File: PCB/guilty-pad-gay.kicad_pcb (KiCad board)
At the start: 2 copper layers, 6 parts

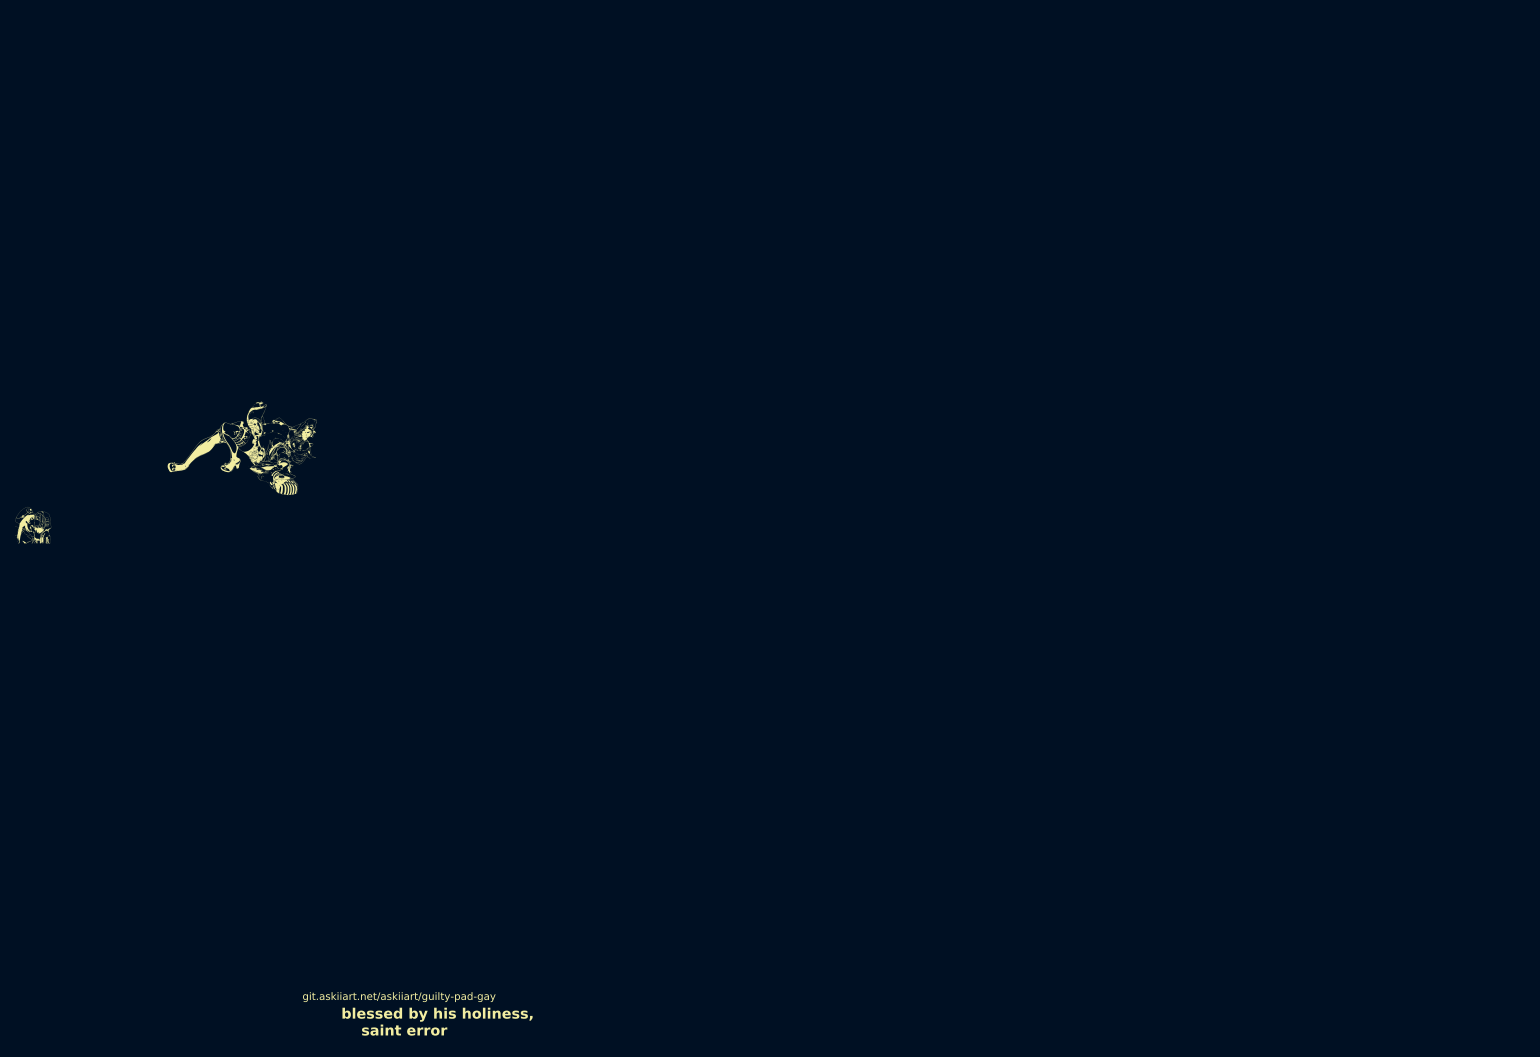
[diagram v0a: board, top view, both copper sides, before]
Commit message: update with routed and parts and stuffs
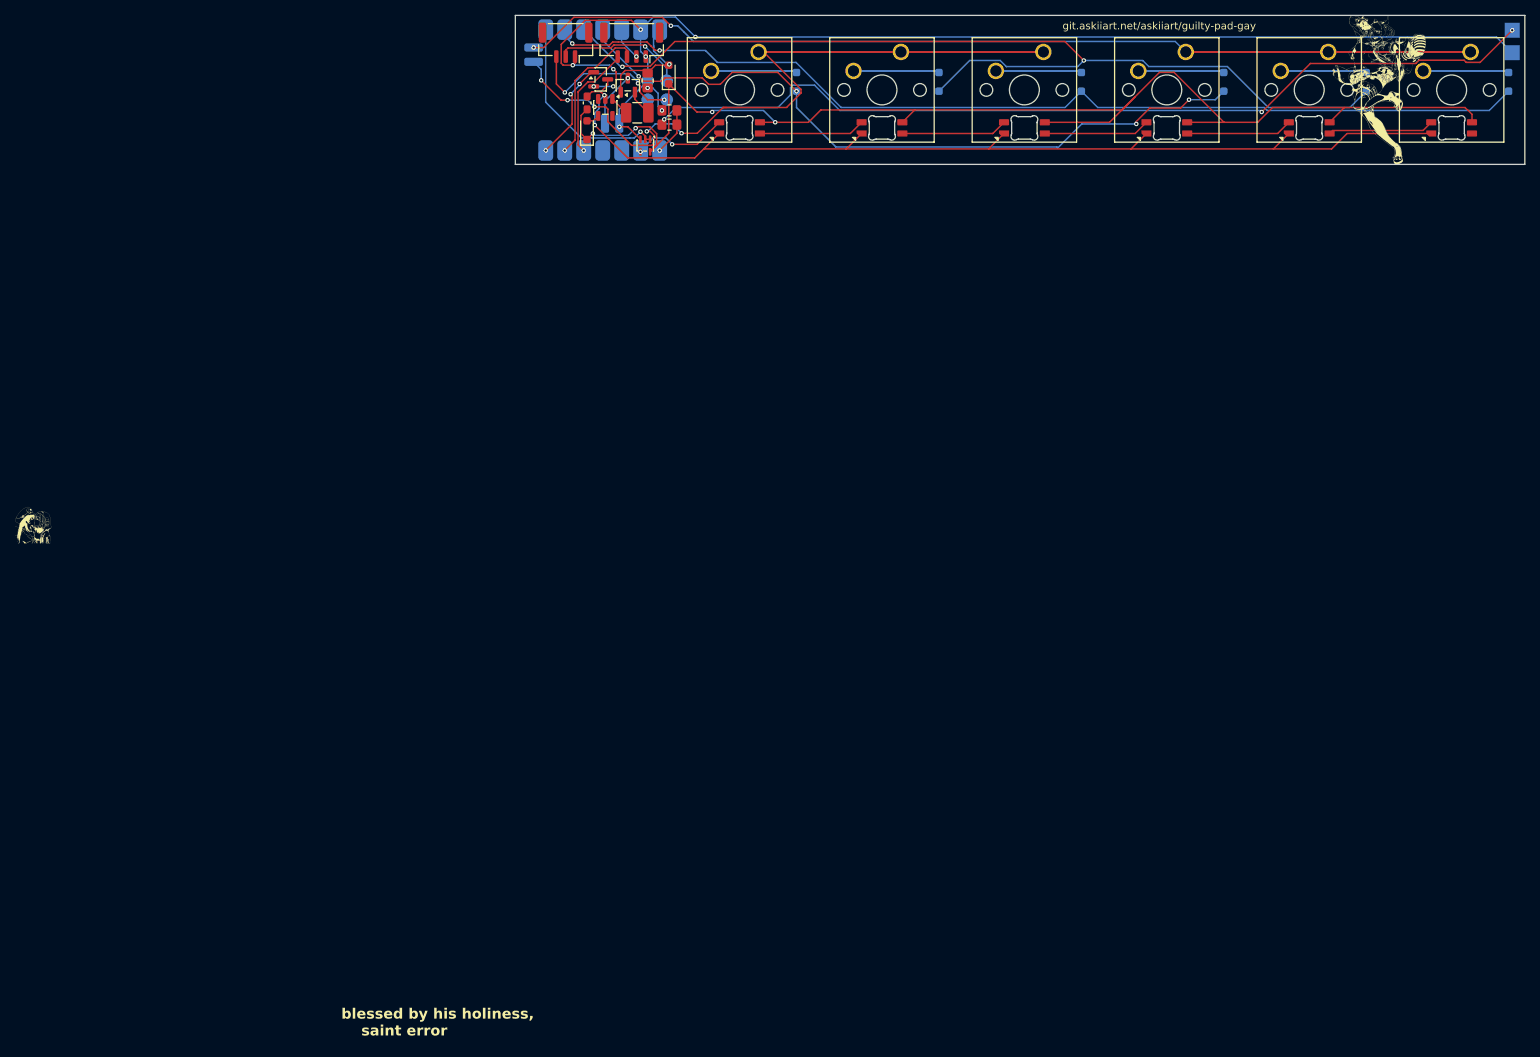
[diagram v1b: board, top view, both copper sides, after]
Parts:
- added C2: 22uF, Capacitor_SMD:C_0603_1608Metric_Pad1.08x0.95mm_HandSolder, F.Cu at (116.0, 70.8)
- added D1: D, Diode_SMD:D_SOD-323_HandSoldering, F.Cu at (116.0, 74.4)
- added D2: D, Diode_SMD:D_SOD-323_HandSoldering, F.Cu at (126.9, 67.0)
- added D3: D_Small, Diode_SMD:D_SOD-323_HandSoldering, B.Cu at (144.0, 68.0)
- added D4: D_Small, Diode_SMD:D_SOD-323_HandSoldering, B.Cu at (201.2, 68.0)
- added D5: D_Small, Diode_SMD:D_SOD-323_HandSoldering, B.Cu at (163.1, 68.0)
- added D6: D_Small, Diode_SMD:D_SOD-323_HandSoldering, B.Cu at (220.2, 68.0)
- added D7: D_Small, Diode_SMD:D_SOD-323_HandSoldering, B.Cu at (182.1, 68.0)
- added D8: D_Small, Diode_SMD:D_SOD-323_HandSoldering, B.Cu at (239.3, 68.0)
- added J1: Conn_01x03, Connector_JST:JST_GH_SM03B-GHS-TB_1x03-1MP_P1.25mm_Horizontal, F.Cu at (113.2, 62.7)
- added J2: Conn_01x04, Connector_JST:JST_GH_SM04B-GHS-TB_1x04-1MP_P1.25mm_Horizontal, F.Cu at (122.0, 62.7)
- added L1: 4.7uH, Inductor_SMD:L_1210_3225Metric_Pad1.42x2.65mm_HandSolder, F.Cu at (122.7, 72.1)
- added LED1: SK6812MINI-E, marbastlib-various:LED_6028R, F.Cu at (136.4, 74.1)
- added LED2: SK6812MINI-E, marbastlib-various:LED_6028R, F.Cu at (155.5, 74.1)
- added LED3: SK6812MINI-E, marbastlib-various:LED_6028R, F.Cu at (174.5, 74.1)
- added LED4: SK6812MINI-E, marbastlib-various:LED_6028R, F.Cu at (193.6, 74.1)
- added LED5: SK6812MINI-E, marbastlib-various:LED_6028R, F.Cu at (212.6, 74.1)
- added LED6: SK6812MINI-E, marbastlib-various:LED_6028R, F.Cu at (231.7, 74.1)
- added Q1: AO3400A, Package_TO_SOT_SMD:SOT-23, F.Cu at (117.8, 67.6)
- added Q2: AO3401A, Package_TO_SOT_SMD:SOT-23, F.Cu at (121.5, 68.4)
- added R1: 806k, Resistor_SMD:R_0805_2012Metric_Pad1.20x1.40mm_HandSolder, F.Cu at (127.0, 73.7)
- added R2: 2M, Resistor_SMD:R_0805_2012Metric_Pad1.20x1.40mm_HandSolder, F.Cu at (127.0, 71.8)
- added R3: 806k, Resistor_SMD:R_0805_2012Metric_Pad1.20x1.40mm_HandSolder, F.Cu at (124.1, 67.8)
- added SW1: SW_Push, Button_Switch_Keyboard:SW_Cherry_MX_1.00u_PCB, F.Cu at (138.9, 64.0)
- added SW2: SW_Push, Button_Switch_Keyboard:SW_Cherry_MX_1.00u_PCB, F.Cu at (158.0, 64.0)
- added SW3: SW_Push, Button_Switch_Keyboard:SW_Cherry_MX_1.00u_PCB, F.Cu at (177.0, 64.0)
- added SW4: SW_Push, Button_Switch_Keyboard:SW_Cherry_MX_1.00u_PCB, F.Cu at (196.1, 64.0)
- added SW5: SW_Push, Button_Switch_Keyboard:SW_Cherry_MX_1.00u_PCB, F.Cu at (215.1, 64.0)
- added SW6: SW_Push, Button_Switch_Keyboard:SW_Cherry_MX_1.00u_PCB, F.Cu at (234.2, 64.0)
- added TP1: TestPoint, TestPoint:TestPoint_Pad_2.0x2.0mm, B.Cu at (239.8, 61.1)
- added TP2: TestPoint, TestPoint:TestPoint_Pad_2.0x2.0mm, B.Cu at (239.8, 64.1)
- added U1: XIAO-nRF52840-SMD, OPL:XIAO-nRF52840-SMD, B.Cu at (118.1, 69.0)
- added U2: TPS613222ADBV, Package_TO_SOT_SMD:SOT-23-5, F.Cu at (118.4, 71.4)
- added U3: 74LV1T08GW, Package_TO_SOT_SMD:SOT-353_SC-70-5, F.Cu at (123.8, 76.5)
- moved G*** 159.8 mm to (222.2, 69.0), turned to 0 degrees
- moved G*** 120.2 mm to (187.7, 72.7)
- moved G*** 53.4 mm to (149.1, 73.7)
- moved G*** 44.7 mm to (165.4, 69.9), turned to 0 degrees
- moved G*** 37.4 mm to (113.2, 68.6), turned to 90 degrees
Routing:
- net /COL1: track 0.00 -> 319.4 mm, vias 0 -> 2
- net /COL0: track 0.00 -> 286.3 mm, vias 0 -> 5
- net +5V: track 0.00 -> 171.3 mm, vias 0 -> 4
- net GND: track 0.00 -> 171.3 mm, vias 0 -> 10
- net /LED_GND: track 0.00 -> 139.5 mm, vias 0 -> 2
- net /ROW1: track 0.00 -> 134.4 mm, vias 0 -> 2
- net /ROW2: track 0.00 -> 134.4 mm, vias 0 -> 2
- net /VBAT: track 0.00 -> 123.0 mm, vias 0 -> 3
- net /ROW0: track 0.00 -> 96.8 mm, vias 0 -> 4
- net Net-(D8-A): track 0.00 -> 69.1 mm
- net Net-(D7-A): track 0.00 -> 69.1 mm
- net Net-(D3-A): track 0.00 -> 69.1 mm
- net Net-(D6-A): track 0.00 -> 69.1 mm
- net Net-(D4-A): track 0.00 -> 69.1 mm
- net Net-(D5-A): track 0.00 -> 69.1 mm
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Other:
- board outline added: 135 x 19.9 mm
